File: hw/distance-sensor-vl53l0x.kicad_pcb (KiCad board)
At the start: 2 copper layers, 24 x 24 mm, 32 parts, among them J1 DFU, J2 USB_OTG, J3 CONN_02X05, J4 UART, U1 STM32F042F6Px, U2 MIC5504-3.3, U3 VL53L0X, U4 MIC5504-2.8

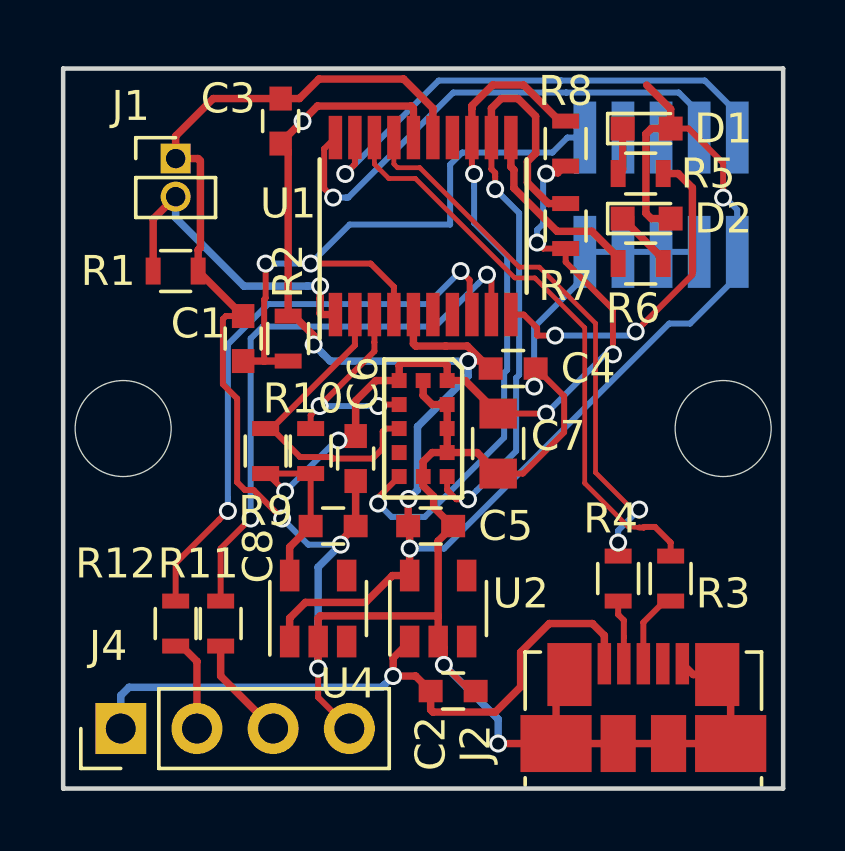
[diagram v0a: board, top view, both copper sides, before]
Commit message: Hardware changes for rev2
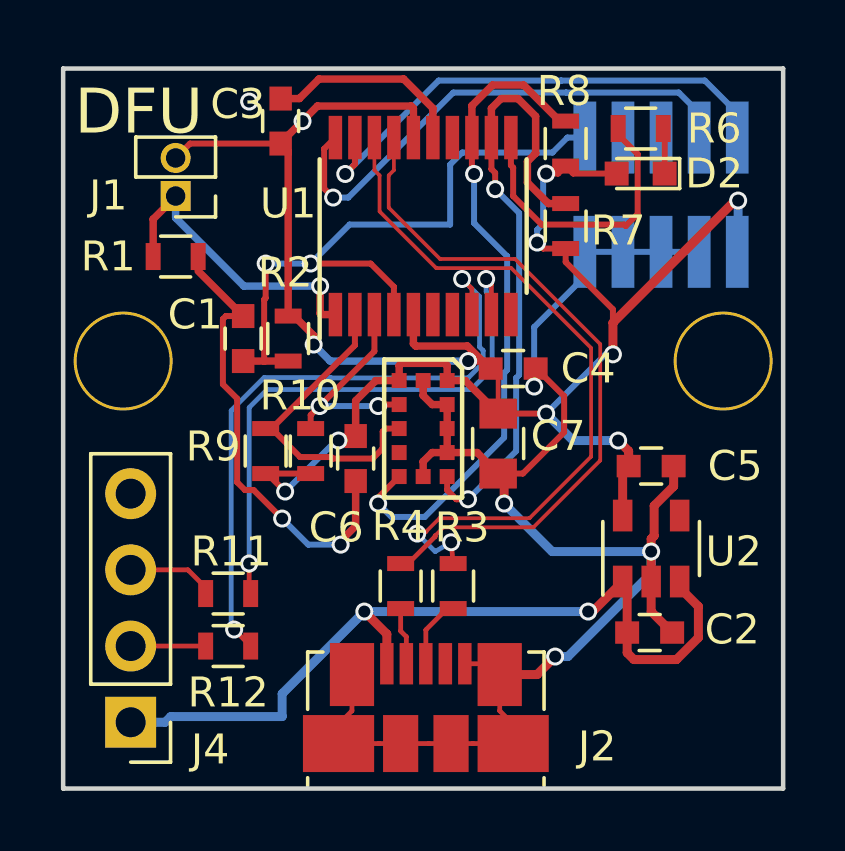
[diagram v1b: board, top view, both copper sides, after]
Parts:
- removed C8: 1uF, Capacitors_SMD:C_0603
- removed D1: LED, LEDs:LED_0603
- removed R5: 220R, Resistors_SMD:R_0603
- removed REF** (x2): MountingHole_3.2mm_M3, Mounting_Holes:MountingHole_3.2mm_M3
- removed U4: MIC5504-2.8, TO_SOT_Packages_SMD:SOT-23-5
- added J101: TEST_1P, mounting_hole:Mounting_hole_3mm, F.Cu at (96.0, 99.8)
- added J102: TEST_1P, mounting_hole:Mounting_hole_3mm, F.Cu at (116.0, 99.8)
- moved C5 7.62 mm to (113.6, 103.2)
- moved U2 7.38 mm to (113.6, 106.0)
- moved R3 7.25 mm to (107.0, 107.2)
- moved R4 7.25 mm to (105.2, 107.2)
- moved J2 7.25 mm to (106.1, 111.2)
- moved C2 6.83 mm to (113.5, 108.8)
- moved R6 4.50 mm to (113.2, 92.0)
- moved R12 1.90 mm to (99.5, 109.2), turned to 180 degrees
- moved D2 1.51 mm to (113.2, 93.5), turned to 180 degrees
- moved J1 1.25 mm to (97.8, 94.2), turned to 180 degrees
- moved R11 1.03 mm to (99.5, 107.5), turned to 180 degrees
- moved R1 0.48 mm to (97.8, 96.3)
- moved J4 0.39 mm to (96.2, 111.8), turned to 180 degrees
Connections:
- C6 pad 1: +2.8V -> +3.3V
- C7 pad 1: +2.8V -> +3.3V
- J1 pad 1: GND -> /BOOT0
- J1 pad 2: /BOOT0 -> +3.3V
- J2 pad 4: (no net) -> Net-(J2-Pad4)
- J3 pad 6: (no net) -> /SWO
- J3 pad 8: (no net) -> Net-(J3-Pad8)
- R10 pad 1: +2.8V -> +3.3V
- R7 pad 1: +2.8V -> +3.3V
- R8 pad 1: +2.8V -> +3.3V
- R9 pad 1: +2.8V -> +3.3V
- U1 pad 14: (no net) -> Net-(U1-Pad14)
- U1 pad 6: (no net) -> Net-(U1-Pad6)
- U1 pad 7: (no net) -> /USART_DE
- U2 pad 3: (no net) -> +5V
- U3 pad 1: +2.8V -> +3.3V
- U3 pad 11: +2.8V -> +3.3V
- U3 pad 8: (no net) -> Net-(U3-Pad8)
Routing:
- net +2.8V: track 30.1 -> 0.00 mm, vias 6 -> 0
- net GND: track 90.9 -> 75.3 mm, vias 6 -> 7
- net Net-(U1-Pad10): track 11.4 -> 0.00 mm, vias 2 -> 0
- net +3.3V: track 63.5 -> 71.4 mm, vias 6 -> 11
- net +5V: track 22.7 -> 28.2 mm, vias 1 -> 2
- net /USB_D_P: track 19.5 -> 24.1 mm, vias 0 -> 2
- net /USB_D_N: track 18.9 -> 23.3 mm, vias 2 -> 0
- net Net-(R6-Pad2): track 6.36 -> 9.83 mm
- net /USART_TX: track 19.7 -> 21.7 mm
- net Net-(D1-Pad1): track 1.56 -> 0.00 mm
- net Net-(J4-Pad2): track 3.16 -> 2.50 mm
- net Net-(D2-Pad1): track 2.06 -> 1.52 mm
- net Net-(J4-Pad3): track 3.47 -> 2.94 mm
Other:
- net class Default: clearance 0.2 -> 0
- rule trace_clearance: 0.2 -> 0
- board text added: "3.3V UART"
- board text added: "DFU"
- board text added: "VCC"
- board text added: "rev2"
- board text removed: "3.3-5.5V in 3.3V IO"
- board text removed: "V+"
